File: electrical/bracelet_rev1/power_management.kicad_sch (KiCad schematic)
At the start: 32 parts, among them J1 USB_C_Receptacle_USB2.0_14P, J3 Conn_01x02, Q1 PMOS, Q2 PMOS, U3 MCP73831T-2ACI/OT, U4 XC6222B331MR-G, U6 TPS62A01DRL, U8 INA180A1

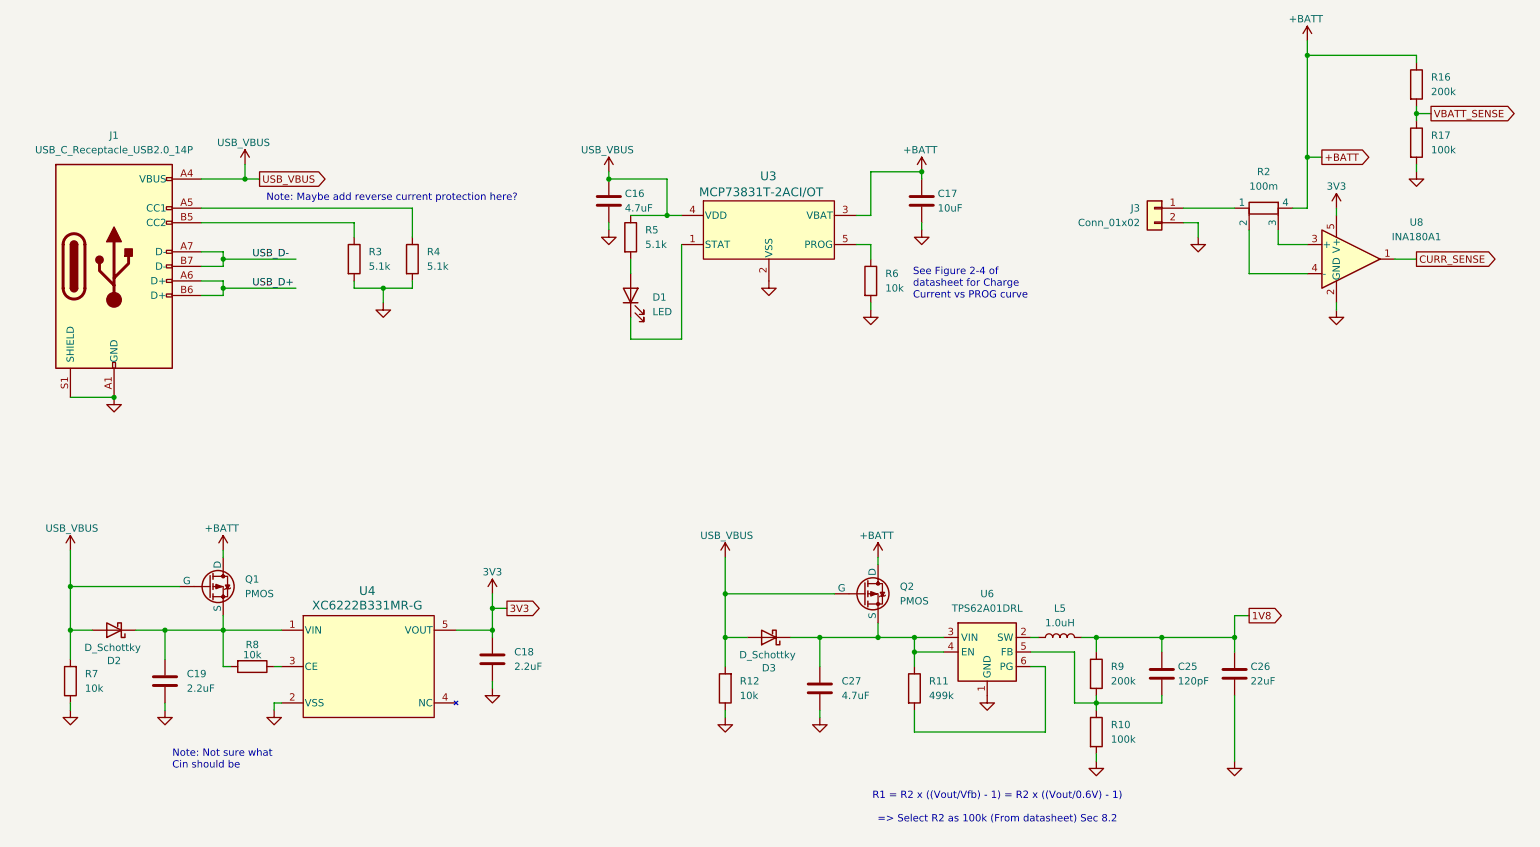
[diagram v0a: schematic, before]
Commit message: May updates
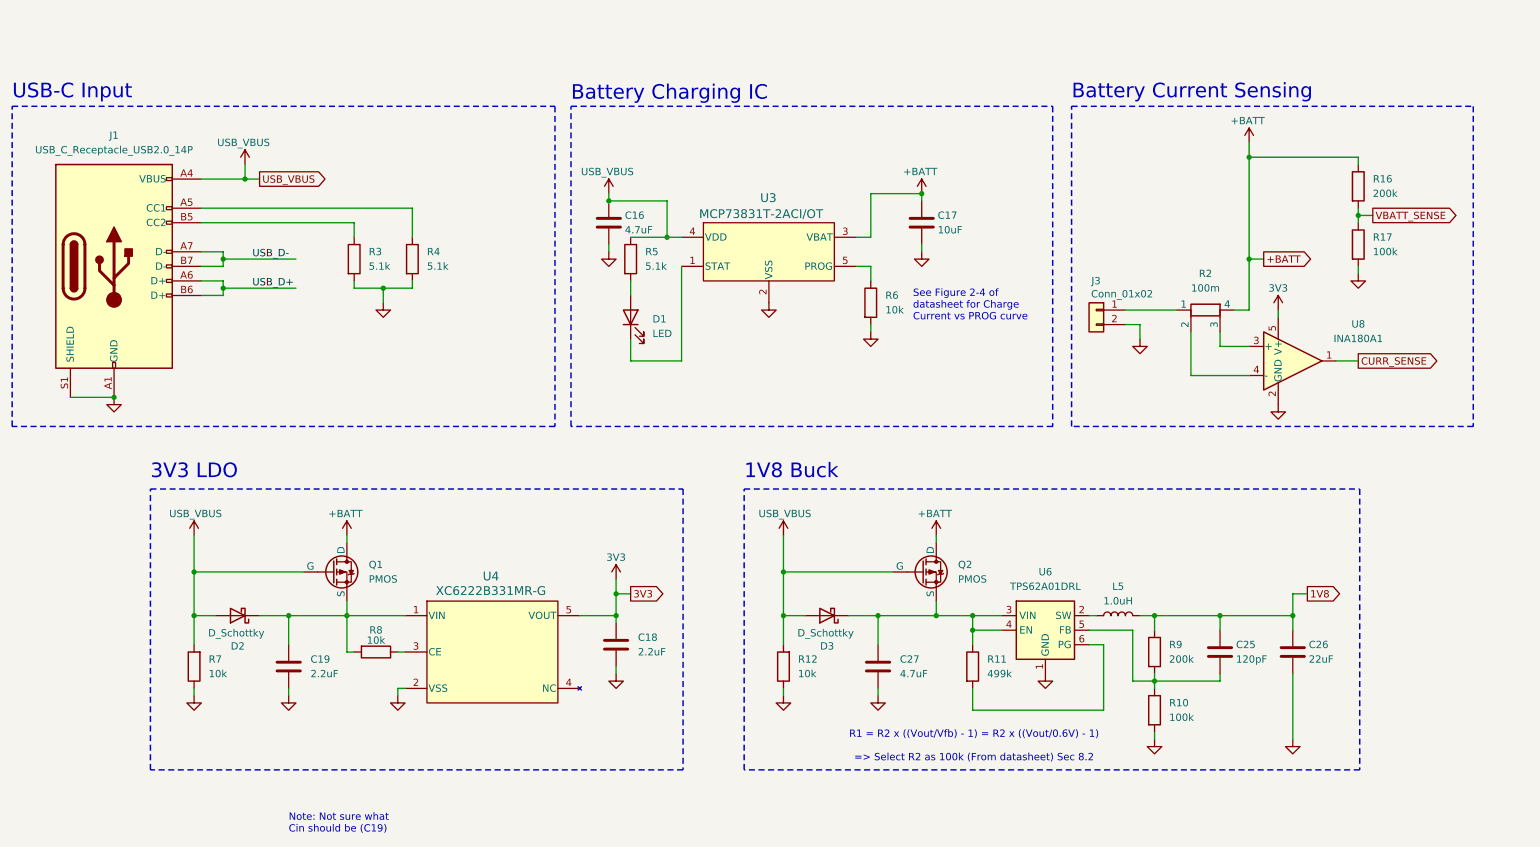
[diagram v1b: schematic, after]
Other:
- note added: "1V8 Buck"
- note added: "3V3 LDO"
- note added: "Battery Charging IC"
- note added: "Battery Current Sensing"
- note added: "Note: Not sure what Cin should be (C19)"
- note added: "USB-C Input"
- note removed: "Note: Maybe add reverse current protection here?"
- note removed: "Note: Not sure what Cin should be"
- moved on the sheet: C16, C17, C18, C19, C25, C26, C27, D1, D2, D3, J3, L5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
